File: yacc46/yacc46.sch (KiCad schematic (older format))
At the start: 142 parts, among them J1 USB_C_Receptacle_USB2.0, J2 OLED_I2C, J3 joystick_switch_joycon, J4 AVR-ISP-6, J5 GLOVE_I2C, SW1 SW_PUSH, SW10 SW_PUSH, SW11 SW_PUSH, SW12 SW_PUSH, SW13 SW_PUSH, SW14 SW_PUSH, SW15 SW_PUSH, SW16 SW_PUSH, SW17 SW_PUSH, SW18 SW_PUSH, SW19 Rotary_Encoder_Switch, SW2 SW_PUSH, SW20 SW_PUSH, SW21 SW_PUSH, SW22 SW_PUSH, SW23 SW_PUSH, SW24 SW_PUSH, SW25 SW_PUSH, SW26 SW_PUSH, SW27 SW_PUSH, SW28 SW_PUSH, SW29 SW_PUSH, SW3 SW_PUSH, SW30 SW_PUSH, SW31 SW_PUSH, SW32 SW_PUSH, SW33 SW_PUSH, SW34 SW_PUSH, SW35 SW_PUSH, SW36 Rotary_Encoder_Switch, SW37 SW_PUSH, SW38 SW_PUSH, SW39 SW_PUSH, SW4 SW_PUSH, SW40 SW_PUSH, SW41 SW_PUSH, SW42 SW_PUSH, SW43 SW_PUSH, SW44 SW_PUSH, SW45 SW_PUSH, SW46 SW_PUSH, SW47 SW_Push, SW5 SW_PUSH, SW6 SW_PUSH, SW7 SW_PUSH, SW8 SW_PUSH, SW9 SW_PUSH, U1 ATmega32U4-AU, Y1 16MHz

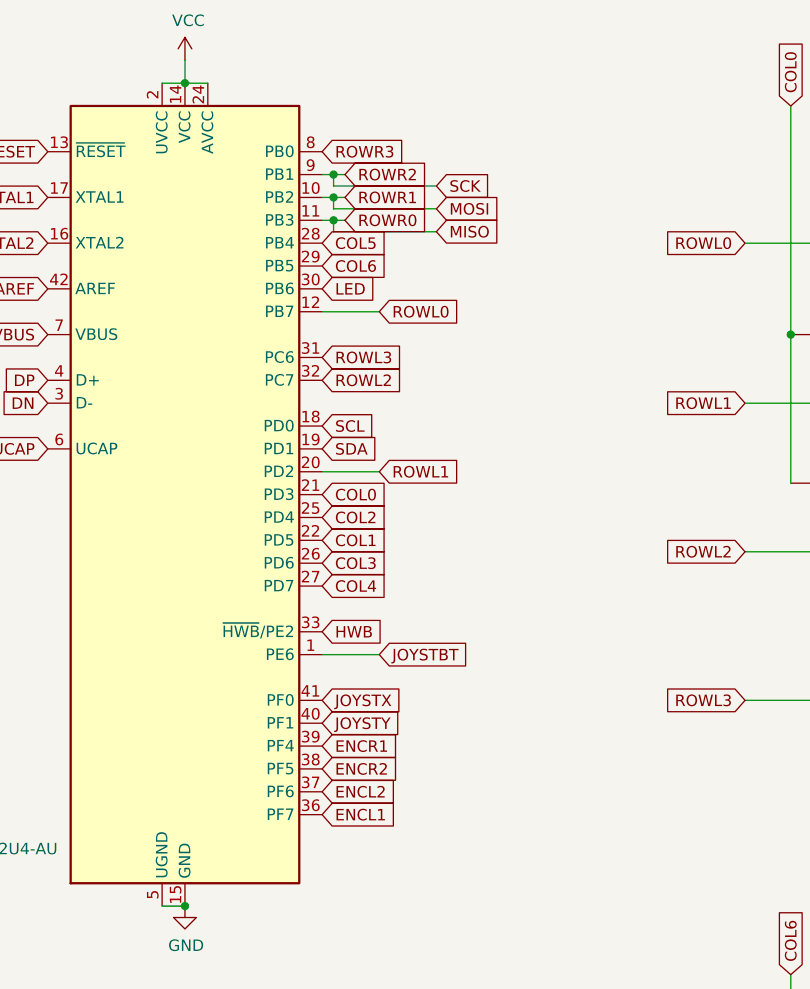
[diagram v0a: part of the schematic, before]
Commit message: 配線完了
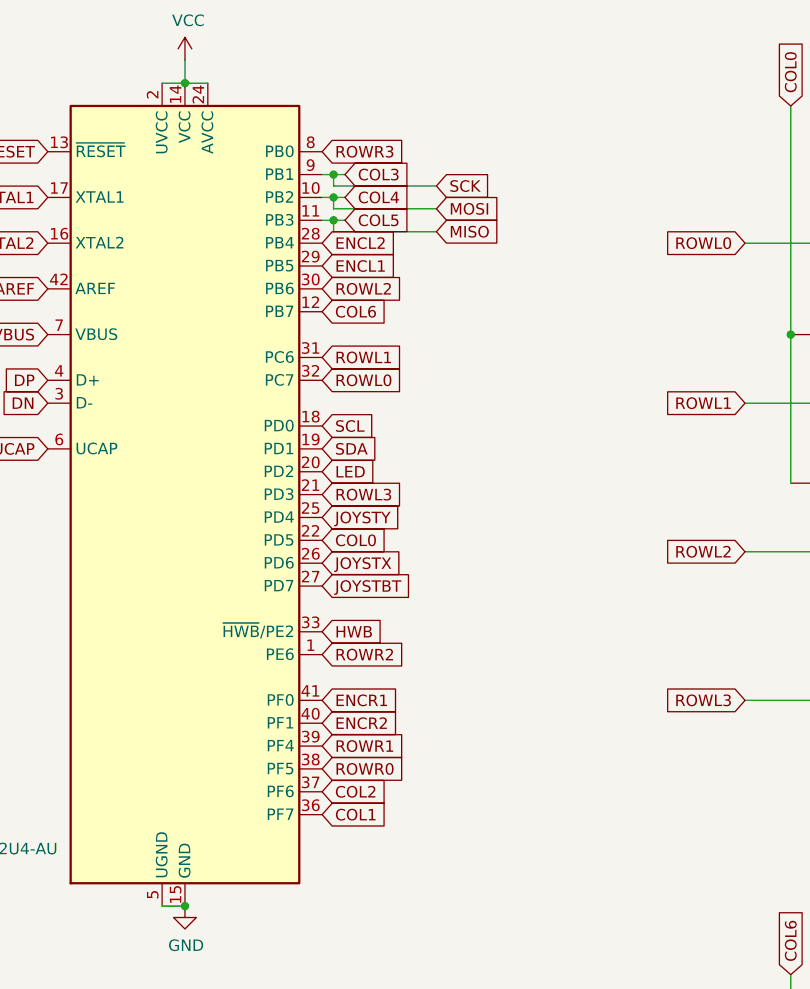
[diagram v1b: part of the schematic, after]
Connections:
- net COL0: now also U1.22 (PD5); no longer U1.21 (PD3)
- net COL1: now also U1.36 (PF7); no longer U1.22 (PD5)
- net COL2: now also U1.37 (PF6); no longer U1.25 (PD4)
- net COL3: now also J4.3 (SCK), U1.9 (PB1); no longer U1.26 (PD6)
- net COL4: now also J4.4 (MOSI), U1.10 (PB2); no longer U1.27 (PD7)
- net COL5: now also J4.1 (MISO), U1.11 (PB3); no longer U1.28 (PB4)
- net COL6: now also U1.12 (PB7); no longer U1.29 (PB5)
- net ENCL1: now also U1.29 (PB5); no longer U1.36 (PF7)
- net ENCL2: now also U1.28 (PB4); no longer U1.37 (PF6)
- net ENCR1: now also U1.41 (PF0); no longer U1.39 (PF4)
- net ENCR2: now also U1.40 (PF1); no longer U1.38 (PF5)
- net JOYSTBT: now also U1.27 (PD7); no longer U1.1 (PE6)
- net JOYSTX: now also U1.26 (PD6); no longer U1.41 (PF0)
- net JOYSTY: now also U1.25 (PD4); no longer U1.40 (PF1)
- net LED: now also U1.20 (PD2); no longer U1.30 (PB6)
- net ROWL0: now also U1.32 (PC7); no longer U1.12 (PB7)
- net ROWL1: now also U1.31 (PC6); no longer U1.20 (PD2)
- net ROWL2: now also U1.30 (PB6); no longer U1.32 (PC7)
- net ROWL3: now also U1.21 (PD3); no longer U1.31 (PC6)
- net ROWR2: now also U1.1 (PE6); no longer J4.3 (SCK), U1.9 (PB1)
- net MISO renamed ROWR0
- net ROWR0: now also U1.38 (PF5); no longer J4.1 (MISO), U1.11 (PB3)
- net MOSI renamed ROWR1
- net ROWR1: now also U1.39 (PF4); no longer J4.4 (MOSI), U1.10 (PB2)
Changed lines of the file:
@@
 Wire Wire Line
 	6400 1600 6400 1650
-Text GLabel 6350 2800 2    50   Input ~ 0
+Text GLabel 6350 3000 2    50   Input ~ 0
 COL0
-Text GLabel 6350 3000 2    50   Input ~ 0
+Text GLabel 6350 4200 2    50   Input ~ 0
 COL1
-Text GLabel 6350 2900 2    50   Input ~ 0
+Text GLabel 6350 4100 2    50   Input ~ 0
 COL2
-Text GLabel 6350 3100 2    50   Input ~ 0
+Text GLabel 6450 1400 2    50   Input ~ 0
 COL3
-Text GLabel 6350 3200 2    50   Input ~ 0
+Text GLabel 6450 1500 2    50   Input ~ 0
 COL4
+Text GLabel 6450 1600 2    50   Input ~ 0
+COL5
+Text GLabel 6350 2000 2    50   Input ~ 0
+COL6
+Text GLabel 6350 3700 2    50   Input ~ 0
+ENCR1
+Text GLabel 6350 3800 2    50   Input ~ 0
+ENCR2
+Text GLabel 6350 1800 2    50   Input ~ 0
+ENCL1
 Text GLabel 6350 1700 2    50   Input ~ 0
-COL5
-Text GLabel 6350 1800 2    50   Input ~ 0
-COL6
-Text GLabel 6350 3900 2    50   Input ~ 0
-ENCR1
-Text GLabel 6350 4000 2    50   Input ~ 0
-ENCR2
-Text GLabel 6350 4200 2    50   Input ~ 0
-ENCL1
-Text GLabel 6350 4100 2    50   Input ~ 0
 ENCL2
-Text GLabel 6350 1900 2    50   Input ~ 0
+Text GLabel 6350 2700 2    50   Input ~ 0
 LED
 Wire Wire Line
@@
 Wire Wire Line
 	3200 8950 3200 8900
-Text GLabel 6450 1600 2    50   Input ~ 0
+Text GLabel 6350 4000 2    50   Input ~ 0
 ROWR0
 Text GLabel 6350 1300 2    50   Input ~ 0
 ROWR3
-Text GLabel 6450 1400 2    50   Input ~ 0
+Text GLabel 6350 3500 2    50   Input ~ 0
 ROWR2
-Text GLabel 6450 1500 2    50   Input ~ 0
+Text GLabel 6350 3900 2    50   Input ~ 0
 ROWR1
-Text GLabel 6600 2700 2    50   Input ~ 0
+Text GLabel 6350 2200 2    50   Input ~ 0
 ROWL1
+Text GLabel 6350 1900 2    50   Input ~ 0
+ROWL2
+Text GLabel 6350 2800 2    50   Input ~ 0
+ROWL3
+Wire Wire Line
+	8200 7500 9000 7500
 Text GLabel 6350 2300 2    50   Input ~ 0
-ROWL2
-Text GLabel 6350 2200 2    50   Input ~ 0
-ROWL3
-Wire Wire Line
-	8200 7500 9000 7500
-Text GLabel 6600 2000 2    50   Input ~ 0
 ROWL0
 Text GLabel 6850 1650 2    50   Input ~ 0
@@
 Wire Wire Line
 	6100 7950 6500 7950
-Text GLabel 6350 3700 2    50   Input ~ 0
+Text GLabel 6350 3100 2    50   Input ~ 0
 JOYSTX
 Text GLabel 6500 8100 0    50   Input ~ 0
 JOYSTX
-Text GLabel 6350 3800 2    50   Input ~ 0
+Text GLabel 6350 2900 2    50   Input ~ 0
 JOYSTY
 Text GLabel 6500 7650 0    50   Input ~ 0
 JOYSTY
-Wire Wire Line
-	6350 2000 6600 2000
-Wire Wire Line
-	6350 2700 6600 2700
-Text GLabel 6600 3500 2    50   Input ~ 0
+Text GLabel 6350 3200 2    50   Input ~ 0
 JOYSTBT
-Wire Wire Line
-	6350 3500 6600 3500
 Text GLabel 6500 7800 0    50   Input ~ 0
 JOYSTBT
